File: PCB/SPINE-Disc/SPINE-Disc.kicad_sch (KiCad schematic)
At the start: 28 parts, among them Q1 NTMFS5C628NLT1G, Q2 NTMFS5C628NLT1G, Q3 NTMFS5C628NLT1G, U1 LM311, U3 TL431DBZ

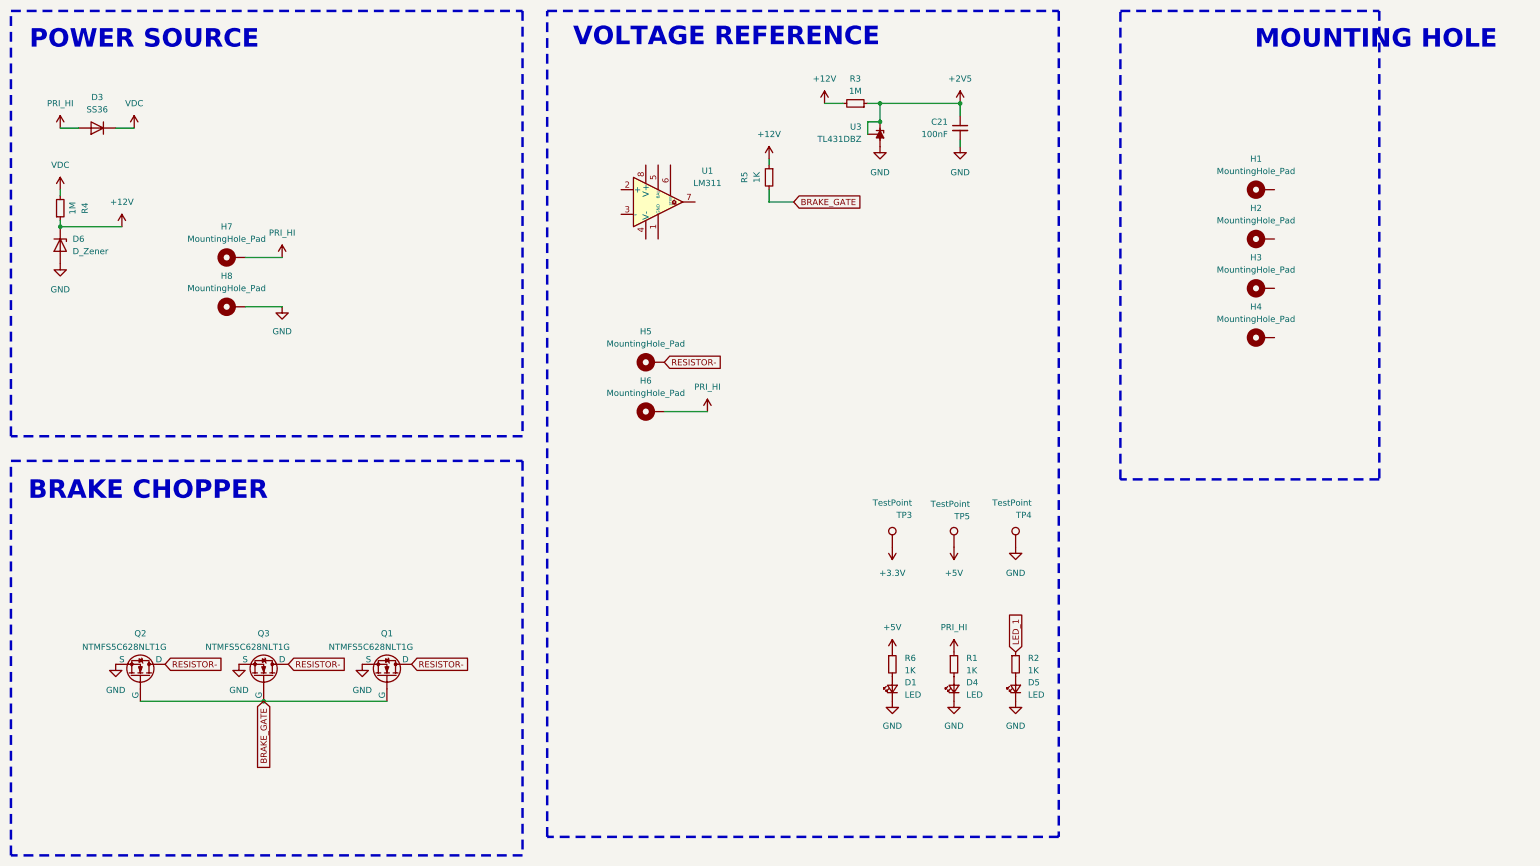
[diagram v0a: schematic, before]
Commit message: update
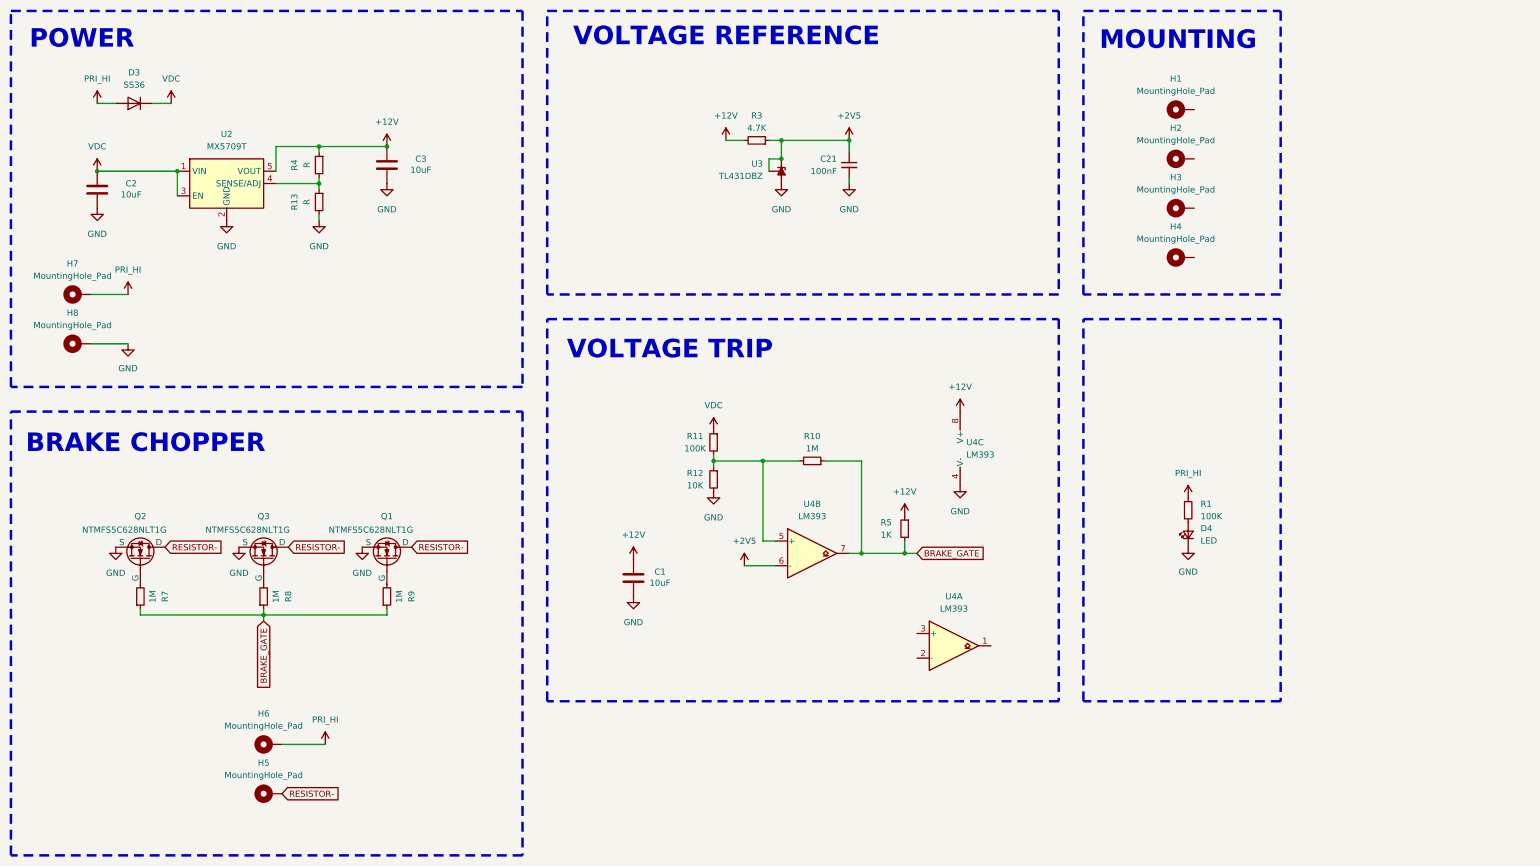
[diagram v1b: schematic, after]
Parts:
- removed D1, D5: LED, LED_SMD:LED_0603_1608Metric, symbol Device:LED_Small
- removed D6: D_Zener, Diode_SMD:D_SOD-323, symbol Device:D_Zener
- removed R2, R6: 1K, Resistor_SMD:R_0603_1608Metric, symbol Device:R_Small
- removed TP3, TP4, TP5: TestPoint, TestPoint:TestPoint_Pad_D1.0mm, symbol Connector:TestPoint
- removed U1: LM311, Package_SO:SOIC-8_3.9x4.9mm_P1.27mm, symbol Comparator:LM311
- added C1, C2, C3: 10uF, Capacitor_SMD:C_1206_3216Metric, symbol Device:C
- added R10, R7, R8, R9: 1M, Resistor_SMD:R_0603_1608Metric, symbol Device:R_Small
- added R11: 100K, Resistor_SMD:R_0603_1608Metric, symbol Device:R_Small
- added R12: 10K, Resistor_SMD:R_0603_1608Metric, symbol Device:R_Small
- added R13: R, Resistor_SMD:R_0603_1608Metric, symbol Device:R_Small
- added U2: MX5709T, Package_TO_SOT_SMD:TSOT-23-5, symbol Regulator_Linear:ADP7142AUJZ
- added U4: LM393, Package_SO:SOIC-8_3.9x4.9mm_P1.27mm, symbol Comparator:LM393
- R1: value 1K -> 100K
- R3: value 1M -> 4.7K
- R4: value 1M -> R
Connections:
- net +12V: now also C1.2, C3.2, U2.5 (VOUT), U4.8 (V+)
- net +2V5: now also U4.6 (-)
- net BRAKE_GATE: now also R10.1, R7.1, R8.1, R9.1, U4.7; no longer Q1.4 (G), Q2.4 (G), Q3.4 (G)
- net GND: now also C1.1, C2.1, C3.1, R12.2, R13.2, U2.2 (GND), U4.4 (V-)
- net VDC: now also C2.2, R11.1, U2.1 (VIN), U2.3 (EN); no longer R4.2
- new net: Q2.4 (G), R7.2
- new net: R10.2, R11.2, R12.1, U4.5 (+)
- new net: Q3.4 (G), R8.2
- new net: R13.1, R4.2, U2.4 (SENSE/ADJ)
- new net: Q1.4 (G), R9.2
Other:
- note added: "MOUNTING"
- note added: "POWER"
- note added: "VOLTAGE TRIP"
- note removed: "MOUNTING HOLE"
- note removed: "POWER SOURCE"
- moved on the sheet: C21, D3, D4, H1, H2, H3, H4, H5, H6, H7, H8, Q1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
